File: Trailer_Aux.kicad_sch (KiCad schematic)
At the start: 14 parts, among them Q44 IRF4905PBF, Q68 2N7000, SW11 KSD9700, SW7 SW_SPST, U12 LM339

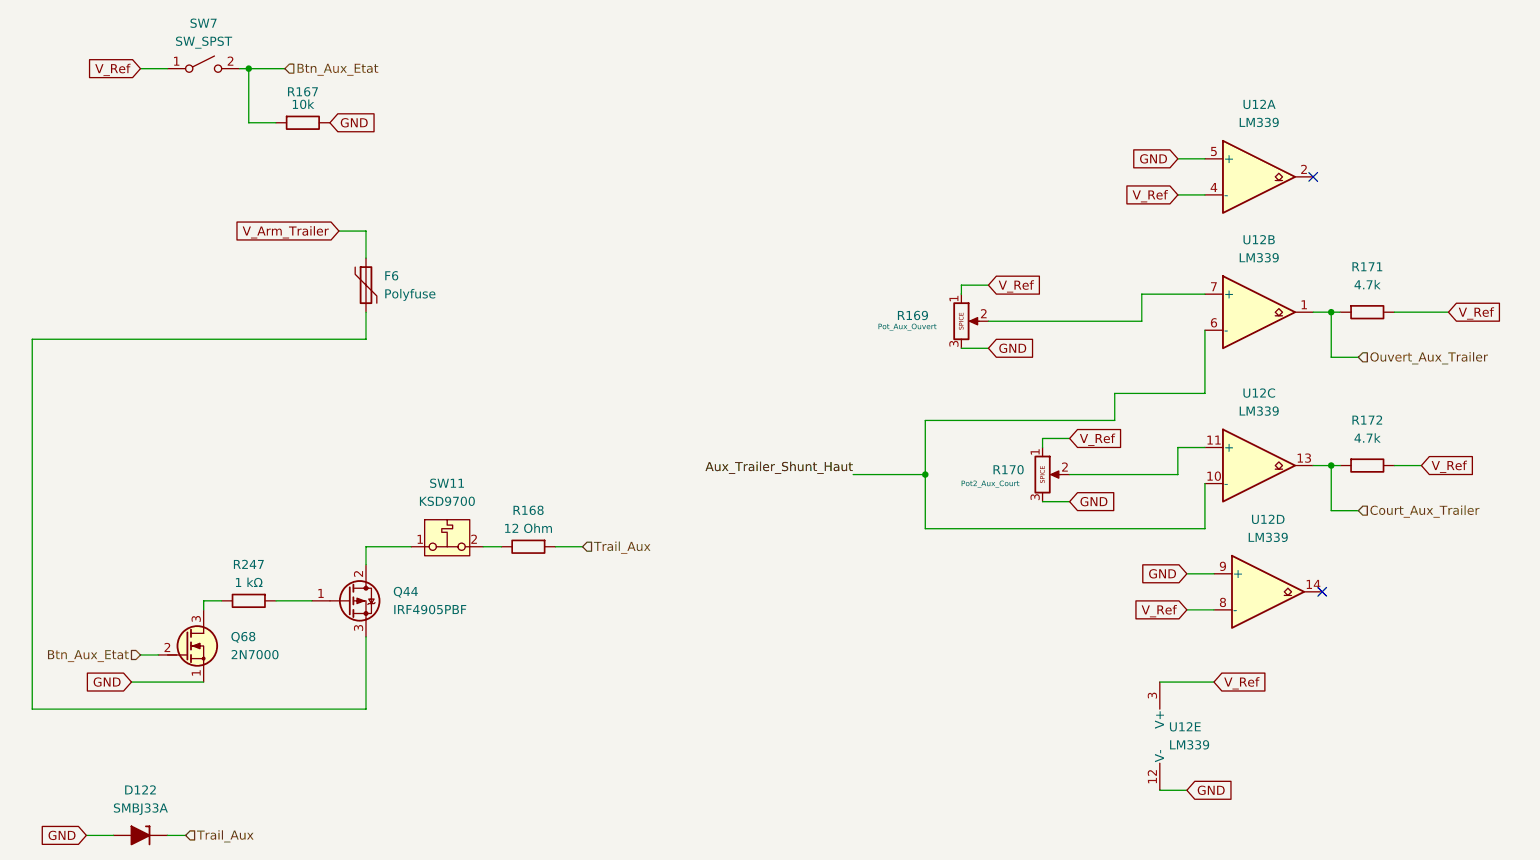
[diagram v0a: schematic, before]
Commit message: Add files via upload
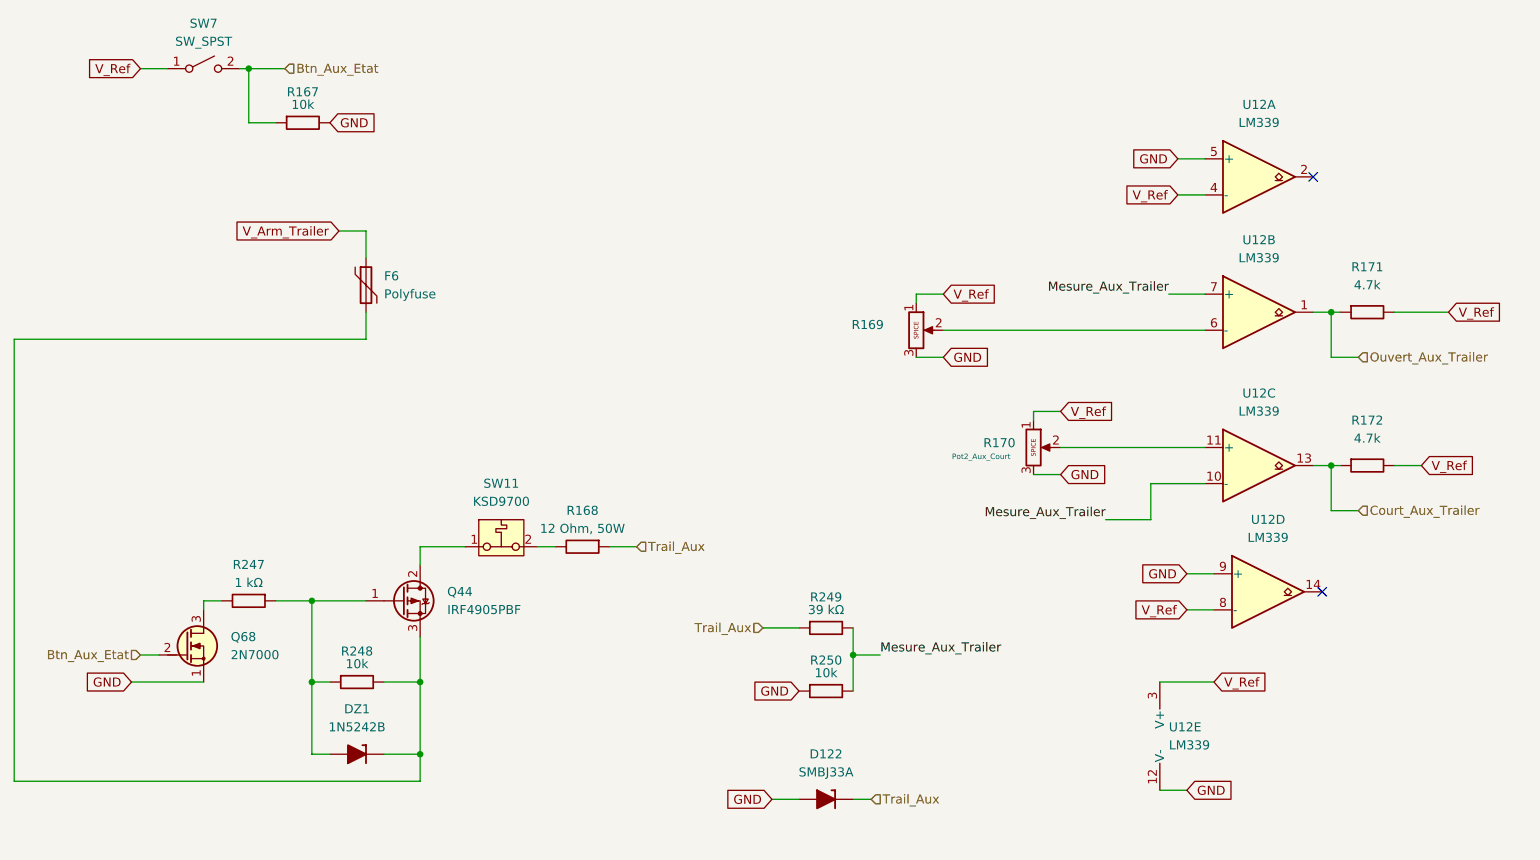
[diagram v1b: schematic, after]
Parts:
- added DZ1: 1N5242B, PCM_Diode_THT_AKL:D_DO-35_SOD27_P7.62mm_Horizontal_Zener, symbol PCM_Diode_Zener_AKL:1N5242B
- added R248, R250: 10k, Resistor_THT:R_Axial_DIN0207_L6.3mm_D2.5mm_P10.16mm_Horizontal, symbol PCM_SL_Resistors:10k
- added R249: 39 kΩ, Resistor_THT:R_Axial_DIN0207_L6.3mm_D2.5mm_P10.16mm_Horizontal, symbol PCM_SL_Resistors:10k
- R168: value 12 Ohm -> 12 Ohm, 50W
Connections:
- net GND: now also R250.1
- net Trail_Aux: now also R249.1
- net at Q44.1 (G), R247.1: now also DZ1.2 (A), R248.1
- net at F6.2, Q44.3 (S): now also DZ1.1 (K), R248.2
- net at R169.2: now also U12.6 (-); no longer U12.7 (+)
- net Aux_Trailer_Shunt_Haut renamed Mesure_Aux_Trailer
- net Mesure_Aux_Trailer: now also U12.7 (+), R249.2, R250.2; no longer U12.6 (-)
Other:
- moved on the sheet: D122, Q44, R168, R169, R170, SW11
